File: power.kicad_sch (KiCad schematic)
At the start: 35 parts, among them U11 AP2114H-3.3TRG1, U15 AMS1117-3.3, U5 INA226, U7 TPS54560DDAR, U9 TPS7A2033DQNR

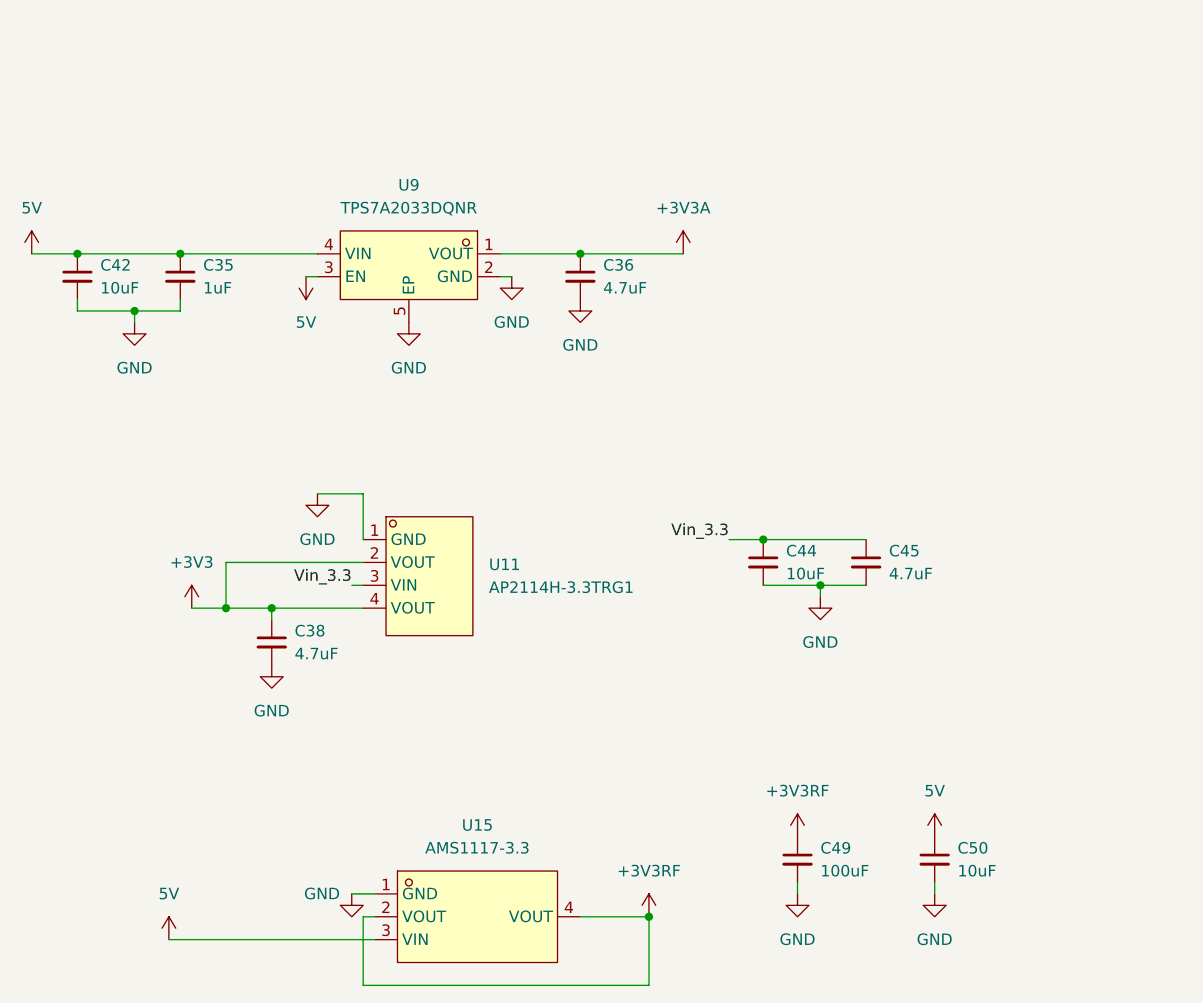
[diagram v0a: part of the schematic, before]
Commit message: finalized RF
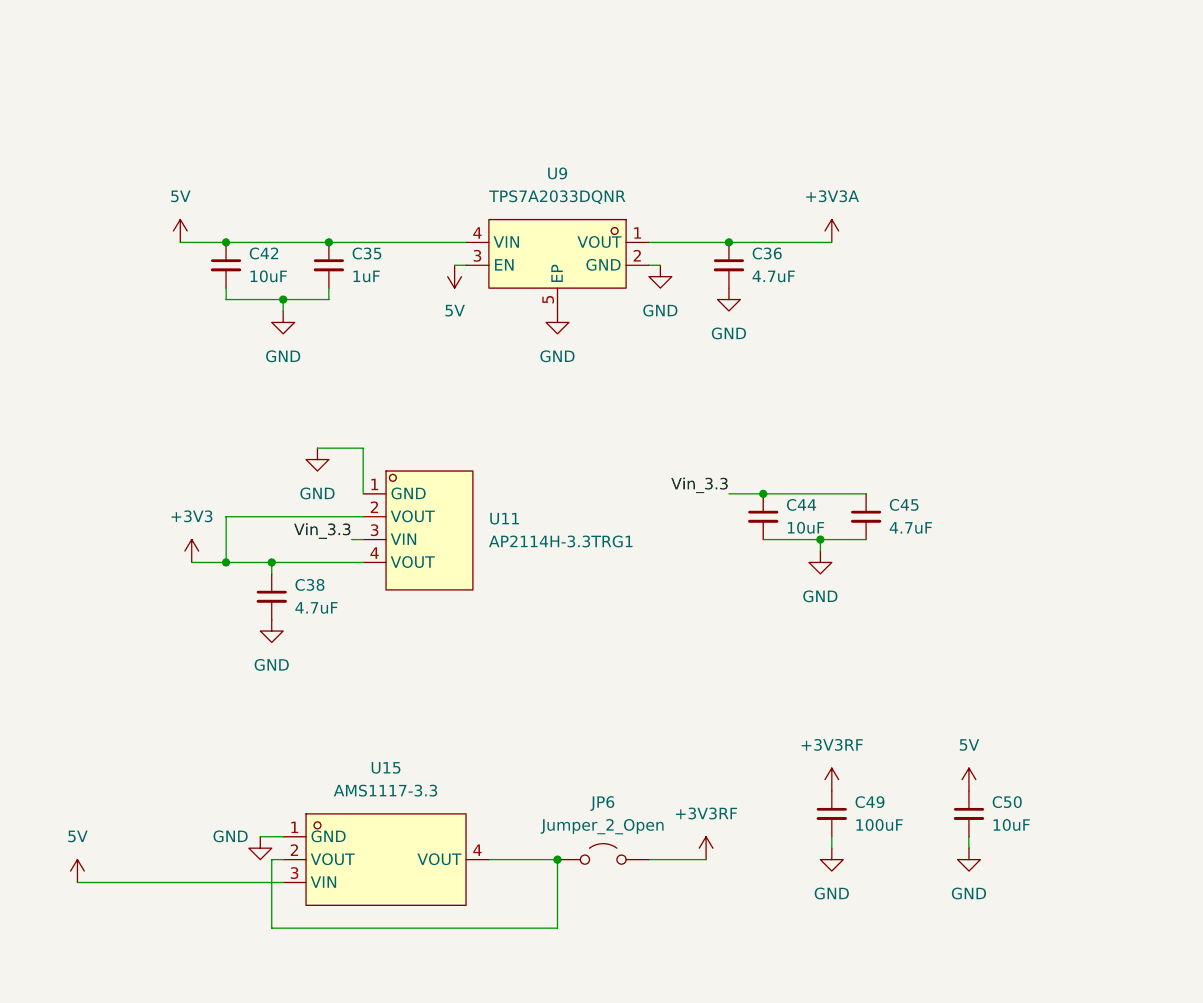
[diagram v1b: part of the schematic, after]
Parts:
- added JP6: Jumper_2_Open, symbol Jumper:Jumper_2_Open
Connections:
- net +3V3RF: now also JP6.2 (B); no longer U15.2 (VOUT), U15.4 (VOUT)
- new net: JP6.1 (A), U15.2 (VOUT), U15.4 (VOUT)
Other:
- moved on the sheet: C35, C36, C38, C42, C44, C45, C49, C50, U11, U15, U9
